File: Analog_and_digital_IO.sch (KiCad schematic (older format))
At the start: 7 parts

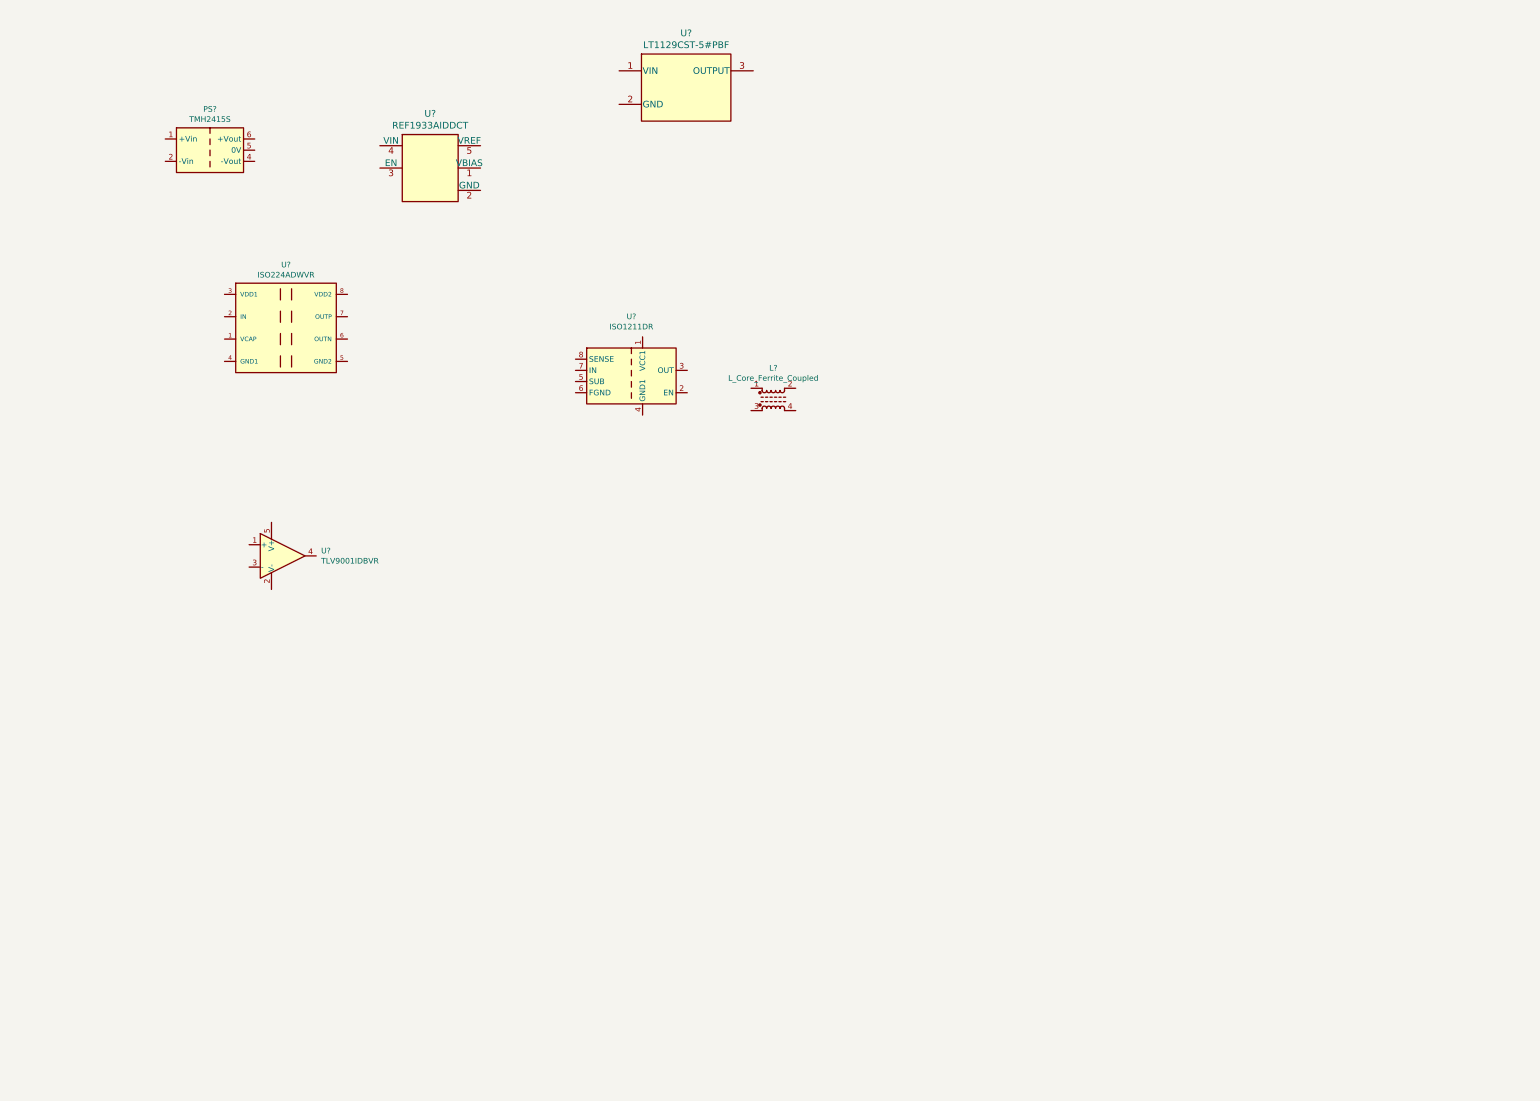
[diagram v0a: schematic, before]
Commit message: Analog Input edited
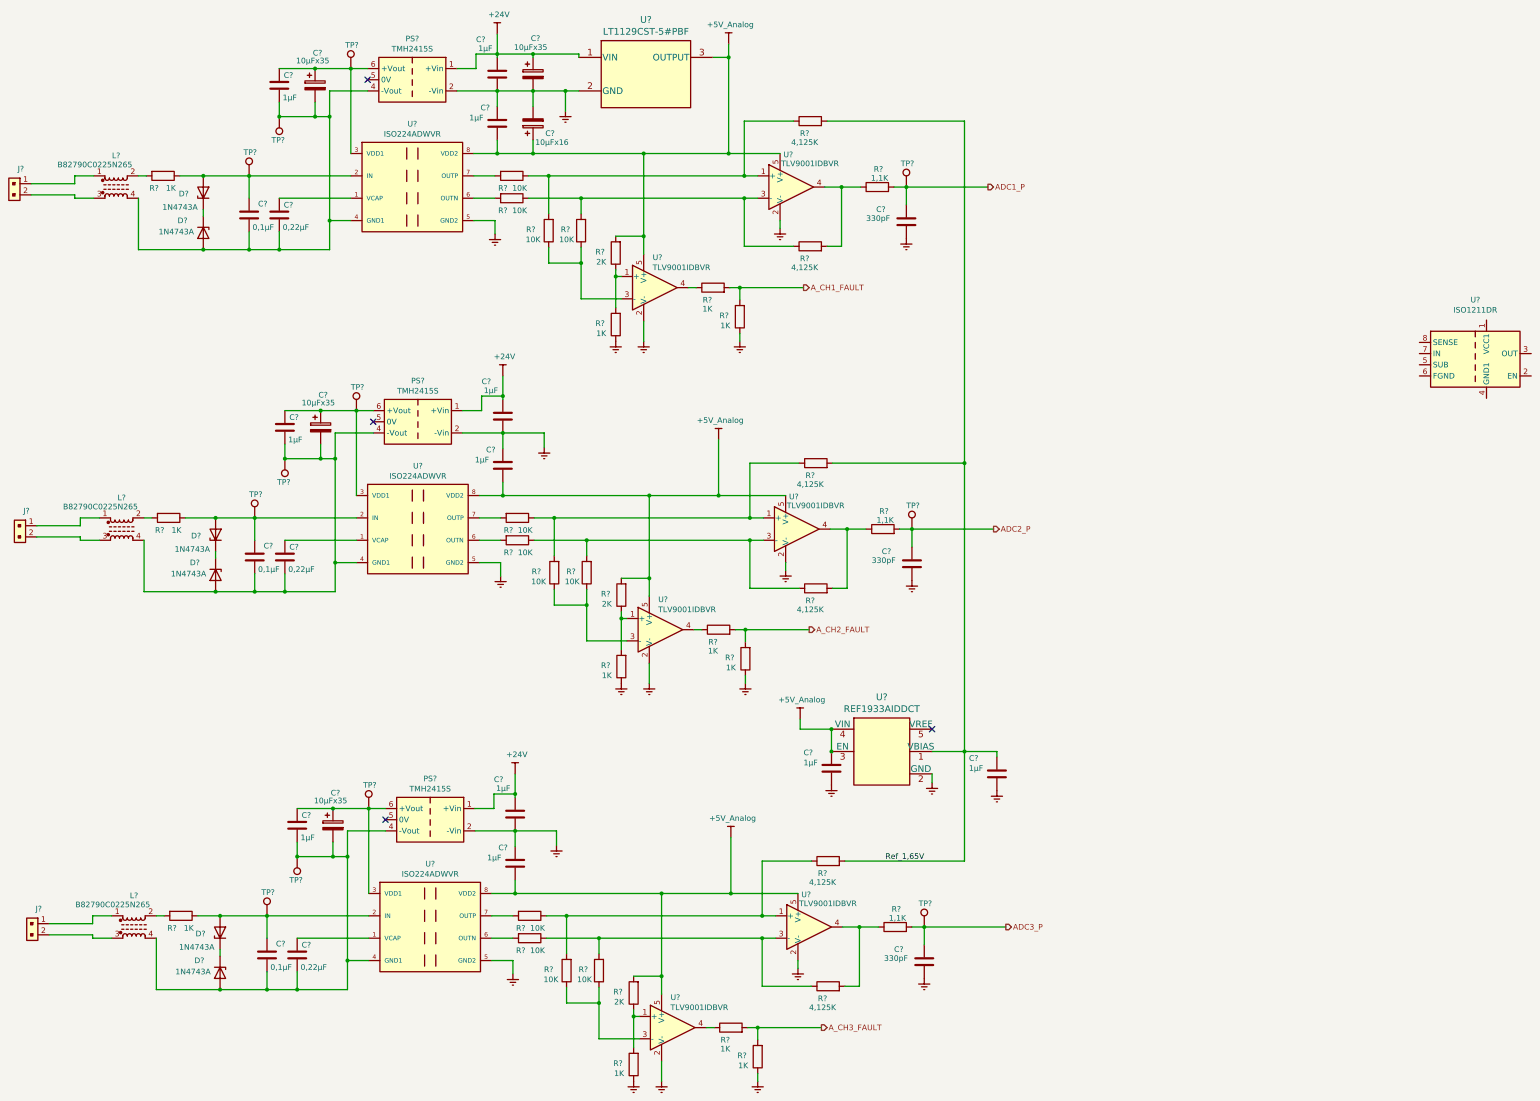
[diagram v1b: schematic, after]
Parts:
- removed U?: LT1129CST-5#PBF, Package_TO_SOT_SMD:SOT-223-3_TabPin2, symbol SVIELCOM_Library:LT1129CST-5#PBF
- removed U?: REF1933AIDDCT, Package_TO_SOT_SMD:SOT-23-5_HandSoldering, symbol SVIELCOM_Library:REF1933AIDDCT
- added C? (x3): 0,22µF, Capacitor_SMD:C_0603_1608Metric_Pad1.08x0.95mm_HandSolder, symbol Device:C
- added C? (x3): 0,1µF, Capacitor_SMD:C_0603_1608Metric_Pad1.08x0.95mm_HandSolder, symbol Device:C
- added C? (x4): 10µFx35, symbol Device:CP
- added C? (x11): 1µF, Capacitor_SMD:C_0603_1608Metric_Pad1.08x0.95mm_HandSolder, symbol Device:C
- added C?: 10µFx16, symbol Device:CP
- added C? (x3): 330pF, Capacitor_SMD:C_0603_1608Metric_Pad1.08x0.95mm_HandSolder, symbol Device:C
- added D? (x6): 1N4743A, Diode_THT:D_DO-41_SOD81_P10.16mm_Horizontal, symbol Diode:1N47xxA
- added J? (x3): 22-23-2021, digikey-footprints:PinHeader_1x2_P2.54mm_Drill1.02mm, symbol dk_Rectangular-Connectors-Headers-Male-Pins:22-23-2021
- added L? (x2): B82790C0225N265, Inductor_SMD:L_Wuerth_WE-DD-Typ-L-Typ-XL-Typ-XXL, symbol Device:L_Core_Ferrite_Coupled
- added PS? (x2): TMH2415S, Converter_DCDC:Converter_DCDC_XP_POWER-IAxxxxS_THT, symbol Converter_DCDC:IA2415S
- added R? (x12): 1K, Resistor_SMD:R_0805_2012Metric_Pad1.20x1.40mm_HandSolder, symbol Device:R
- added R? (x12): 10K, Resistor_SMD:R_0805_2012Metric_Pad1.20x1.40mm_HandSolder, symbol Device:R
- added R? (x3): 2K, Resistor_SMD:R_0805_2012Metric_Pad1.20x1.40mm_HandSolder, symbol Device:R
- added R? (x6): 4,125K, Resistor_SMD:R_0805_2012Metric_Pad1.20x1.40mm_HandSolder, symbol Device:R
- added R? (x3): 1,1K, Resistor_SMD:R_0805_2012Metric_Pad1.20x1.40mm_HandSolder, symbol Device:R
- added TP? (x12): TestPoint, symbol Connector:TestPoint
- added U?: LT1129CST-5#PBF, Package_TO_SOT_SMD:SOT-223-3_TabPin2, symbol SVIELCOM_Library:LT1129CST-5#PBF
- added U?: REF1933AIDDCT, Package_TO_SOT_SMD:SOT-23-5_HandSoldering, symbol SVIELCOM_Library:REF1933AIDDCT
- added U? (x5): TLV9001IDBVR, Package_TO_SOT_SMD:SOT-23-5_HandSoldering, symbol Amplifier_Operational:TLV9001IDCK
- added U? (x2): ISO224ADWVR, Texas_Instruments-DWV0008A-0-0-*, symbol Схема-и-печатная-плата-rescue:ISO224ADWVR-Isolator
- L?: value L_Core_Ferrite_Coupled -> B82790C0225N265
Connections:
- net +24V: now reaches PS?.1 (+Vin)
- net +24V: now also C?.1, C?.1, C?.1, C?.1, PS?.1 (+Vin), PS?.1 (+Vin), U?.1 (VIN)
- net GNDREF: now reaches PS?.2 (-Vin)
- net GNDREF: now also U?.2 (V-), U?.5 (GND2), C?.1, C?.1, C?.1, C?.2, C?.2, C?.2, C?.2, C?.2, C?.2, C?.2, C?.2, C?.2, C?.2, PS?.2 (-Vin), PS?.2 (-Vin), R?.1, R?.1, R?.1, R?.1, R?.1, R?.1, U?.2 (GND), U?.2 (GND), U?.2 (V-), U?.2 (V-), U?.2 (V-), U?.2 (V-), U?.2 (V-), U?.5 (GND2), U?.5 (GND2)
- net at PS?.4 (-Vout): now also L?.4, U?.4 (GND1), C?.2, C?.2, C?.2, C?.2, D?.2 (A), TP?.1
- net at PS?.6 (+Vout): now also U?.3 (VDD1), C?.1, C?.1, TP?.1
- net at L?.1: now also J?.1
- net at L?.2: now also R?.2
- net at L?.3: now also J?.2
- net at U?.1 (VCAP): now also C?.1
- net at U?.2 (IN): now also C?.1, D?.2 (A), R?.1, TP?.1
- net at U?.6 (OUTN): now also R?.2
- net at U?.7 (OUTP): now also R?.2
- net +5V_Analog: now reaches U?.8 (VDD2)
- net +5V_Analog: now also U?.5 (V+), C?.1, C?.1, C?.2, C?.2, C?.2, R?.2, R?.2, R?.2, U?.3 (EN), U?.3 (OUTPUT), U?.4 (VIN), U?.5 (V+), U?.5 (V+), U?.5 (V+), U?.5 (V+), U?.5 (V+), U?.8 (VDD2), U?.8 (VDD2)
- net at U?.1 (+): now also R?.1, R?.2
- net at U?.3 (-): now also R?.1, R?.1
- net at U?.4: now also R?.1
- new net: D?.1 (K), D?.1 (K) (x3)
- new net: R?.1, R?.1, R?.2, U?.1 (+) (x3)
- new net: R?.1, R?.1, R?.2, U?.3 (-) (x3)
- new net: R?.1, R?.2, U?.4 (x3)
- new net: J?.1, L?.1 (x2)
- new net: L?.2, R?.2 (x2)
- new net: J?.2, L?.3 (x2)
- new net: C?.2, C?.2, C?.2, C?.2, D?.2 (A), L?.4, PS?.4 (-Vout), TP?.1, U?.4 (GND1) (x2)
- new net: C?.1, U?.1 (VCAP) (x2)
- new net: C?.1, D?.2 (A), R?.1, TP?.1, U?.2 (IN) (x2)
- new net: C?.1, C?.1, PS?.6 (+Vout), TP?.1, U?.3 (VDD1) (x2)
- new net: R?.2, U?.6 (OUTN) (x2)
- new net: R?.2, U?.7 (OUTP) (x2)
- new net: R?.1, R?.2, U?.1 (+) (x2)
- new net: R?.1, R?.1, U?.3 (-) (x2)
- new net: R?.1, U?.4 (x2)
- new net ADC1_P: C?.1, R?.2, TP?.1
- new net ADC2_P: C?.1, R?.2, TP?.1
- new net ADC3_P: C?.1, R?.2, TP?.1
- new net A_CH1_FAULT: R?.2, R?.2
- new net A_CH2_FAULT: R?.2, R?.2
- new net A_CH3_FAULT: R?.2, R?.2
- new net Ref_1,65V: C?.1, R?.2, R?.2, R?.2, U?.1 (VBIAS)
- no-connect marks 0 -> 4
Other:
- moved on the sheet: L?, PS?, U?
